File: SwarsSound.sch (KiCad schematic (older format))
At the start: 9 parts, among them P1 Main_Connector

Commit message: Add files via upload
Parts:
- added 5F/H, F/H-5: 74LS125, symbol 74xx:74LS125
- added C1, C12, C61, C8, C9: 0.1uf, symbol Device:C
- added H-5: LS74, symbol Star_Wars_Vector_PCB:LS74
- added R1: 1000, symbol Device:R_US
- added R2, R3: 10K, symbol Device:R_US
- F_5: symbol Star_Wars_Audio_PCB:LS161A -> SwarsSound-rescue:LS161A-Star_Wars_Audio_PCB
- gave numbers to parts that had none: 3
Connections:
- net labels added: MAINFLAG, P, SA0, SA1, SA10, SA11, SA12, SA13, SA14, SA2, SA3, SA4, SA5, SA6, SA7, SA8, SA9, SD0, SD1, SD2, SD3, SD4, SD5, SD6, SD7, SOUNDFLAG, SR\~W, S~IRQ, ~SOUNDREAD, ~SOUNDWR, ~SRES, ɸE
- wire segments 143 -> 197
- no-connect marks 43 -> 51
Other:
- note added: "Microprocessor"
- note added: "Parallel Interface with Full Handshaking"
- moved on the sheet: C6, H_2E, J_3B, J_5, K-3, K_5, R4

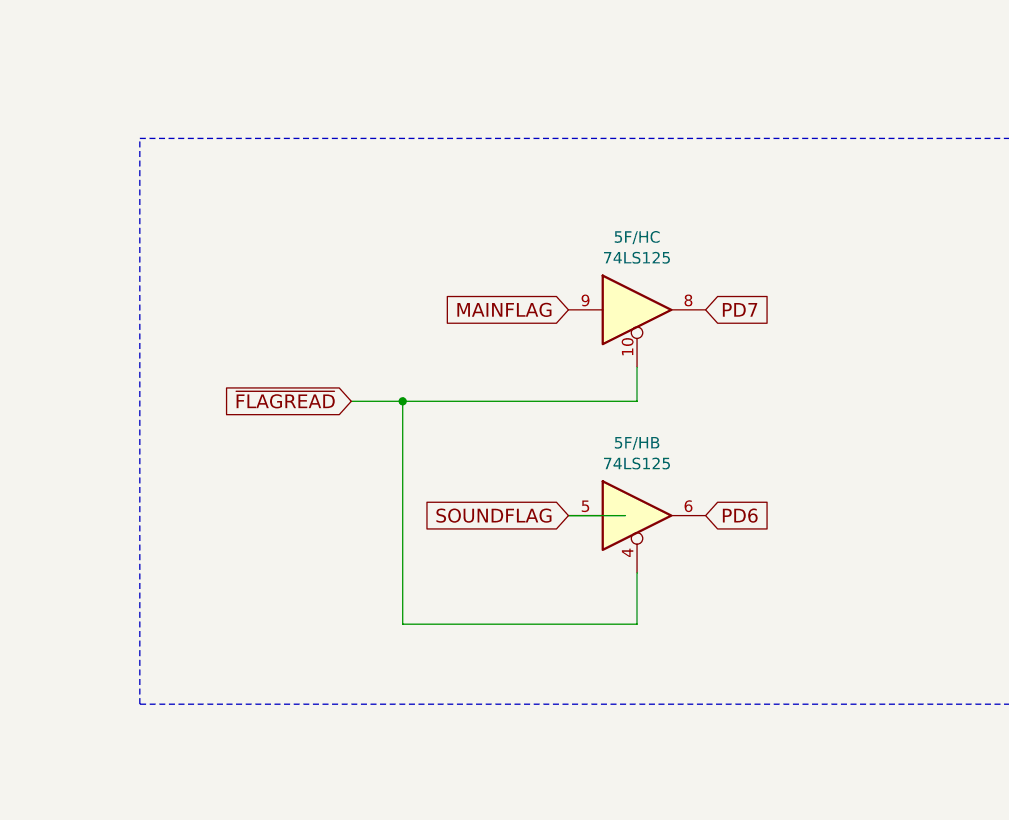
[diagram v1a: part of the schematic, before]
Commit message: Add files via upload
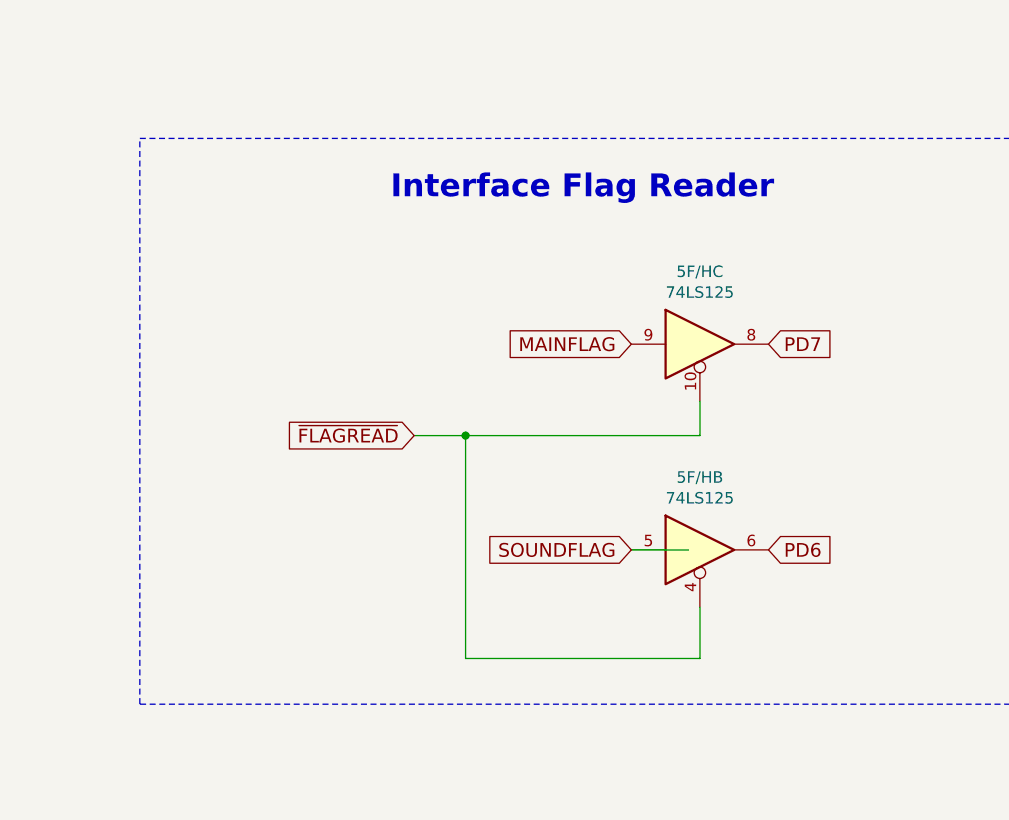
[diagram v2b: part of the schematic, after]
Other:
- note added: "Interface Flag Reader"
- moved on the sheet: 5F/HB, 5F/HC
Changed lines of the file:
@@
 L 74xx:74LS125 5F/H
 U 3 1 60E16230
-P 13400 8250
-F 0 "5F/H" H 13400 8567 50  0000 C CNN
-F 1 "74LS125" H 13400 8476 50  0000 C CNN
-F 2 "" H 13400 8250 50  0001 C CNN
-F 3 "http://www.ti.com/lit/gpn/sn74LS125" H 13400 8250 50  0001 C CNN
-	3    13400 8250
+P 13675 8400
+F 0 "5F/H" H 13675 8717 50  0000 C CNN
+F 1 "74LS125" H 13675 8626 50  0000 C CNN
+F 2 "" H 13675 8400 50  0001 C CNN
+F 3 "http://www.ti.com/lit/gpn/sn74LS125" H 13675 8400 50  0001 C CNN
+	3    13675 8400
 	1    0    0    -1
 $EndComp
@@
 L 74xx:74LS125 5F/H
 U 2 1 60E1786D
-P 13400 9150
-F 0 "5F/H" H 13400 9467 50  0000 C CNN
-F 1 "74LS125" H 13400 9376 50  0000 C CNN
-F 2 "" H 13400 9150 50  0001 C CNN
-F 3 "http://www.ti.com/lit/gpn/sn74LS125" H 13400 9150 50  0001 C CNN
-	2    13400 9150
+P 13675 9300
+F 0 "5F/H" H 13675 9617 50  0000 C CNN
+F 1 "74LS125" H 13675 9526 50  0000 C CNN
+F 2 "" H 13675 9300 50  0001 C CNN
+F 3 "http://www.ti.com/lit/gpn/sn74LS125" H 13675 9300 50  0001 C CNN
+	2    13675 9300
 	1    0    0    -1
 $EndComp
-Text GLabel 13100 8250 0    60   Input ~ 0
+Text GLabel 13375 8400 0    60   Input ~ 0
 MAINFLAG
-Text GLabel 13100 9150 0    60   Input ~ 0
+Text GLabel 13375 9300 0    60   Input ~ 0
 SOUNDFLAG
 Wire Wire Line
-	13350 9150 13100 9150
-Text GLabel 13700 8250 2    60   Input ~ 0
+	13625 9300 13375 9300
+Text GLabel 13975 8400 2    60   Input ~ 0
 PD7
 Wire Wire Line
-	13400 8500 13400 8650
+	13675 8650 13675 8800
 Wire Wire Line
-	13400 8650 12375 8650
-Text GLabel 12150 8650 0    60   Input ~ 0
+	13675 8800 12650 8800
+Text GLabel 12425 8800 0    60   Input ~ 0
 ~FLAGREAD
 Wire Wire Line
-	12375 8650 12375 9625
+	12650 8800 12650 9775
 Wire Wire Line
-	12375 9625 13400 9625
+	12650 9775 13675 9775
 Wire Wire Line
-	13400 9625 13400 9400
-Connection ~ 12375 8650
+	13675 9775 13675 9550
+Connection ~ 12650 8800
 Wire Wire Line
-	12375 8650 12150 8650
-Text GLabel 13700 9150 2    60   Input ~ 0
+	12650 8800 12425 8800
+Text GLabel 13975 9300 2    60   Input ~ 0
 PD6
 Wire Notes Line width 40 style solid rgb(0, 0, 0)
@@
 Wire Notes Line width 40 style solid rgb(0, 0, 0)
 	11225 9975 11225 7500
+Text Notes 14000 7775 2    100  ~ 20
+Interface Flag Reader
 $EndSCHEMATC

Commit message: Joint session
Added footprints and plopped chips on nonexistent board.
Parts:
- removed 5F/H: 74LS125, symbol 74xx:74LS125
- removed F_5: LS161A, symbol SwarsSound-rescue:LS161A-Star_Wars_Audio_PCB
- added A-3: NE556, Star_Wars_Vector_PCB:DIP14, symbol SwarsSound-rescue:NE556-Timer
- added B-2, C-3, C-4: TL084, Star_Wars_Vector_PCB:DIP14, symbol SwarsSound-rescue:TL084-Amplifier_Operational
- added B-3: RD5106A, Star_Wars_Vector_PCB:DIP8, symbol SwarsSound-rescue:RD5106A-Audio
- added C/D-1: TMS-5220, Star_Wars_Main_PCB:DIP28, symbol Star_Wars_Audio_PCB:TMS-5220
- added C10, C11, C16, C17, C18, C19, C2, C20, C28, C3, C4, C5, C7: 0.1uf, Star_Wars_Vector_PCB:GenericComp, symbol Device:C
- added C22, C23, C24, C25, C26, C27, C30, C31, C32, C34, C36, C37, C38, C40, C41, C42, C43, C45, C54, C55, C59, C60: 0.1, Star_Wars_Vector_PCB:GenericComp, symbol Device:C
- added C29, C33, C35, C39: 1000pf, Star_Wars_Vector_PCB:GenericComp, symbol Device:C
- added C44: 0.01, Star_Wars_Vector_PCB:GenericComp, symbol Device:C
- added C46, C48, C49, C50, C56, C57, C58: .0027, Star_Wars_Vector_PCB:GenericComp, symbol Device:C
- added C47, C53: 100, Star_Wars_Vector_PCB:GenericComp, symbol Device:C
- added C51: 0.47, Star_Wars_Vector_PCB:GenericComp, symbol Device:C
- added C52: 10, Star_Wars_Vector_PCB:GenericComp, symbol Device:C
- added D-2: CI/O 3, Package_DIP:DIP-40_W15.24mm, symbol SwarsSound-rescue:POKEY-Star_Wars_Audio_PCB
- added D-3: CI/O 2, Package_DIP:DIP-40_W15.24mm, symbol SwarsSound-rescue:POKEY-Star_Wars_Audio_PCB
- added D-4: CI/O 1, Package_DIP:DIP-40_W15.24mm, symbol SwarsSound-rescue:POKEY-Star_Wars_Audio_PCB
- added D-5: CI/O 0, Package_DIP:DIP-40_W15.24mm, symbol SwarsSound-rescue:POKEY-Star_Wars_Audio_PCB
- added E-1: 6532A PIA, Package_DIP:DIP-40_W15.24mm, symbol SwarsSound-rescue:6532A-Star_Wars_Audio_PCB
- added F-2: CD4069/74C04, Star_Wars_Vector_PCB:DIP14, symbol SwarsSound-rescue:4069-4xxx
- added F-3, F-5: LS161A, Star_Wars_Vector_PCB:DIP16, symbol Star_Wars_Audio_PCB:LS161A
- added F/H-1: 6116-2K-RAM, Star_Wars_Vector_PCB:DDIP24, symbol SwarsSound-rescue:6116-2K-RAM
- added unit 3 of F/H-5
- added unit 2 of F/H-5
- added H-1, J/K-1: 2764, Star_Wars_Main_PCB:DIP28, symbol star_wars_arcade_main_pcb:2764
- added H-2: LS04, Star_Wars_Vector_PCB:DIP14, symbol Star_Wars_Vector_PCB:LS04
- added H-3: LS00, Star_Wars_Vector_PCB:DIP14, symbol Asteroids:LS00
- added J-2: LS139, Star_Wars_Vector_PCB:DIP16, symbol Asteroids:LS139
- added unit 1 of J-3
- added P2: aud_con, Star_Wars_Vector_PCB:Aud_Con_7, symbol Star_Wars_Audio_PCB:aud_con
- added P3: edge_con, Star_Wars_Vector_PCB:J20, symbol Star_Wars_Audio_PCB:edge_con
- added Q1, Q2: 2N3906f, Star_Wars_Vector_PCB:GenericTrans, symbol SwarsSound-rescue:2N3906f-Transistor_BJT
- added Q3, Q4: 2N3904, Package_TO_SOT_THT:TO-92_Inline, symbol Transistor_BJT:2N3904
- added R10, R13, R17, R37, R5, R6: 10K, Star_Wars_Vector_PCB:GenericComp, symbol Device:R_US
- added R11, R14, R16: 3300, Star_Wars_Vector_PCB:GenericComp, symbol Device:R_US
- added R12, R15, R20, R22, R24, R26, R28: 1000, Star_Wars_Vector_PCB:GenericComp, symbol Device:R_US
- added R18: 1800, Star_Wars_Vector_PCB:GenericComp, symbol Device:R_US
- added R19: 100K, Star_Wars_Vector_PCB:GenericComp, symbol Device:R_US
- added R21, R23, R50, R54, R55: 47K, Star_Wars_Vector_PCB:GenericComp, symbol Device:R_US
- added R25, R27: 82K, Star_Wars_Vector_PCB:GenericComp, symbol Device:R_US
- added R29: 15K, Star_Wars_Vector_PCB:GenericComp, symbol Device:R_US
- added R30, R39, R40, R42, R46, R47: 12K, Star_Wars_Vector_PCB:GenericComp, symbol Device:R_US
- added R31, R32: 560K, Star_Wars_Vector_PCB:GenericComp, symbol Device:R_US
- added R33, R34: 4700, Star_Wars_Vector_PCB:GenericComp, symbol Device:R_US
- added R35, R51, R56: 2.2K, Star_Wars_Vector_PCB:GenericComp, symbol Device:R_US
- added R36: 15, Star_Wars_Vector_PCB:GenericComp, symbol Device:R_US
- added R38: 470, Star_Wars_Vector_PCB:GenericComp, symbol Device:R_US
- added R41: 68K, Star_Wars_Vector_PCB:GenericComp, symbol Device:R_US
- added R43: 1500, Star_Wars_Vector_PCB:GenericComp, symbol Device:R_US
- added R44, R8, R9: 100, Star_Wars_Vector_PCB:GenericComp, symbol Device:R_US
- added R45: 470K, Star_Wars_Vector_PCB:GenericComp, symbol Device:R_US
- added R48, R49, R52, R53: 22K, Star_Wars_Vector_PCB:GenericComp, symbol Device:R_US
- added TP1, TP10, TP2, TP7, TP8, TP9: TP, Star_Wars_Vector_PCB:TEST_POINT, symbol Star_Wars_Vector_PCB:TP
- C1, C12, C6, C61, C8, C9, R1, R2, R3, R4: footprint (none) -> Star_Wars_Vector_PCB:GenericComp
- F/H-5, H-5, H_2: footprint (none) -> Star_Wars_Vector_PCB:DIP14
- J-3: renamed from J_3; footprint (none) -> Star_Wars_Vector_PCB:DIP16
- J-5: renamed from J_5; footprint (none) -> Star_Wars_Vector_PCB:DIP20
- K-3: footprint (none) -> Star_Wars_Vector_PCB:DDIP40
- K-5: renamed from K_5; footprint (none) -> Star_Wars_Vector_PCB:DIP20
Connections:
- net labels added: +12V, +5A, -5V, AUD, CO0, CO1, CO2, CO3, DRCV, DXMT, LT_AUD, PA0, PA1, PA2, PA3, PA5, PB0, PB1, PB2, PB3, PB4, PB5, PB6, PB7, RCK, RT_AUD, SPEECH, SUM, ~CI\O, ~CI\O0, ~CI\O1, ~CI\O2, ~CI\O3, ~PIA, ~SRAM, ~SROM0, ~SROM1
- wire segments 197 -> 497
- no-connect marks 51 -> 101
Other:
- note added: "Address Decoders"
- note added: "Buffers"
- note added: "Delay"
- note added: "Delay Clock"
- note added: "Filter"
- note added: "Music and Sound Effects Generators"
- note added: "Not fitted"
- note added: "Output and Summing Amplifiers"
- note added: "Peripheral Interface Adapter"
- note added: "SELF-TEST"
- note added: "Sound RAM\n"
- note added: "Sound ROM"
- note added: "Speech Synthesizer"
- note added: "Speech Synthesizer Clock Generator"
- note added: "Speech Synthesizer Power Switch"
- note added: "Summing Amplifier"
- note added: "Used by buffers"
- moved on the sheet: C1, C6, C8, C9, F/H-5E, H-5B, J-3B, J-5, K-5

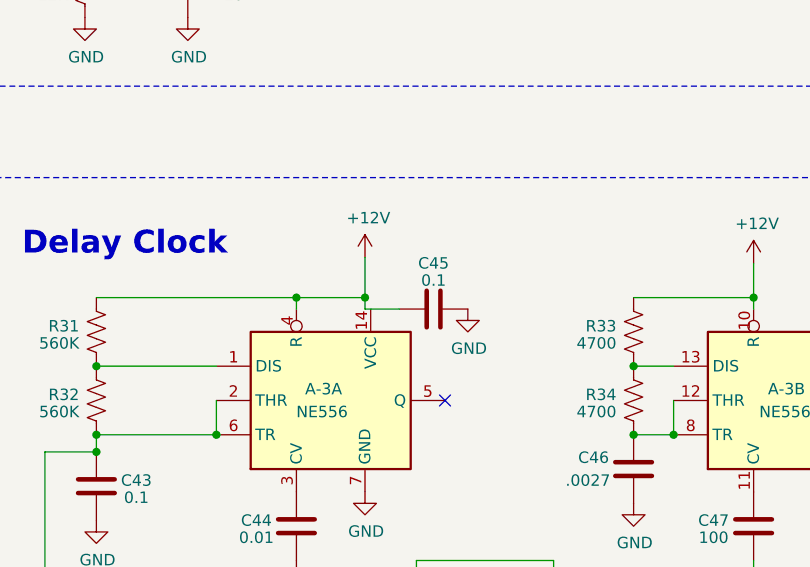
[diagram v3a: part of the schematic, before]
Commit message: Began board layout
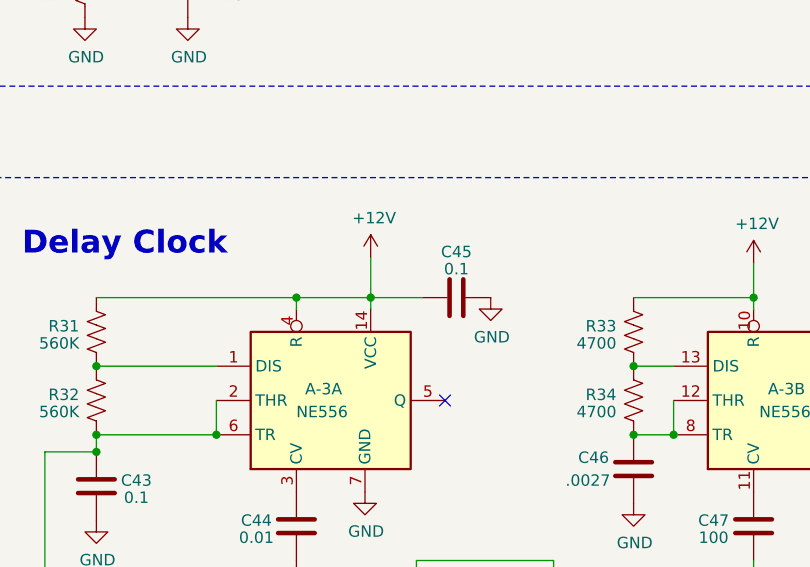
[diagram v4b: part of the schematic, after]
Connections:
- net +12V: now also A-3.14 (VCC)
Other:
- moved on the sheet: C45
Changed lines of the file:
@@
 $EndComp
 NoConn ~ 22575 14550
-Wire Wire Line
-	22375 14150 22225 14150
-Wire Wire Line
-	22225 13925 22225 14100
 $Comp
 L power:GND #PWR0130
 U 1 1 61A178FF
-P 22675 14150
-F 0 "#PWR0130" H 22675 13900 50  0001 C CNN
-F 1 "GND" H 22680 13977 50  0000 C CNN
-F 2 "" H 22675 14150 50  0001 C CNN
-F 3 "" H 22675 14150 50  0001 C CNN
-	1    22675 14150
+P 22775 14100
+F 0 "#PWR0130" H 22775 13850 50  0001 C CNN
+F 1 "GND" H 22780 13927 50  0000 C CNN
+F 2 "" H 22775 14100 50  0001 C CNN
+F 3 "" H 22775 14100 50  0001 C CNN
+	1    22775 14100
 	1    0    0    -1
 $EndComp
-Connection ~ 22225 14100
 $Comp
 L Device:C C45
 U 1 1 619FBD8D
-P 22525 14150
-F 0 "C45" V 22725 14150 50  0000 C CNN
-F 1 "0.1" V 22650 14150 50  0000 C CNN
-F 2 "Star_Wars_Vector_PCB:GenericComp" H 22563 14000 50  0001 C CNN
-F 3 "~" H 22525 14150 50  0001 C CNN
-	1    22525 14150
+P 22625 14100
+F 0 "C45" V 22825 14100 50  0000 C CNN
+F 1 "0.1" V 22750 14100 50  0000 C CNN
+F 2 "Star_Wars_Vector_PCB:GenericComp" H 22663 13950 50  0001 C CNN
+F 3 "~" H 22625 14100 50  0001 C CNN
+	1    22625 14100
 	0    -1   -1   0
 $EndComp
 Connection ~ 21925 14100
 Wire Wire Line
-	22225 14100 22225 14150
-Wire Wire Line
-	21925 14100 22225 14100
+	21925 14100 22250 14100
 Wire Wire Line
 	21925 14100 21925 14150
 Wire Wire Line
 	21050 14100 21925 14100
-Connection ~ 21575 14700
 Wire Wire Line
 	21575 14550 21575 14700
@@
 	1    0    0    -1
 $EndComp
-$Comp
-L SwarsSound-rescue:NE556-Timer A-3
-U 1 1 618D148D
-P 22075 14550
-F 0 "A-3" H 22125 14600 50  0000 R CNN
-F 1 "NE556" H 22150 14500 50  0000 R CNN
-F 2 "Star_Wars_Vector_PCB:DIP14" H 22075 14550 50  0001 C CNN
-F 3 "http://www.ti.com/lit/ds/symlink/ne556.pdf" H 22075 14550 50  0001 C CNN
-	1    22075 14550
-	1    0    0    -1
-$EndComp
 Wire Wire Line
 	22450 15425 22450 15250
@@
 L power:+12V #PWR0236
 U 1 1 61EDFE84
-P 22225 13925
-F 0 "#PWR0236" H 22225 13775 50  0001 C CNN
-F 1 "+12V" H 22240 14098 50  0000 C CNN
-F 2 "" H 22225 13925 50  0001 C CNN
-F 3 "" H 22225 13925 50  0001 C CNN
-	1    22225 13925
+P 22250 13925
+F 0 "#PWR0236" H 22250 13775 50  0001 C CNN
+F 1 "+12V" H 22265 14098 50  0000 C CNN
+F 2 "" H 22250 13925 50  0001 C CNN
+F 3 "" H 22250 13925 50  0001 C CNN
+	1    22250 13925
 	1    0    0    -1
 $EndComp
@@
 	1    0    0    -1
 $EndComp
+Connection ~ 21575 14700
+$Comp
+L SwarsSound-rescue:NE556-Timer A-3
+U 1 1 618D148D
+P 22075 14550
+F 0 "A-3" H 22125 14600 50  0000 R CNN
+F 1 "NE556" H 22150 14500 50  0000 R CNN
+F 2 "Star_Wars_Vector_PCB:DIP14" H 22075 14550 50  0001 C CNN
+F 3 "http://www.ti.com/lit/ds/symlink/ne556.pdf" H 22075 14550 50  0001 C CNN
+	1    22075 14550
+	1    0    0    -1
+$EndComp
+Wire Wire Line
+	22250 13925 22250 14100
+Wire Wire Line
+	22250 14100 22475 14100
+Connection ~ 22250 14100
+Wire Wire Line
+	22250 14150 22250 14100
 $EndSCHEMATC
